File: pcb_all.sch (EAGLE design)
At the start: 1 part, among them IC1 STM32L412KBT6

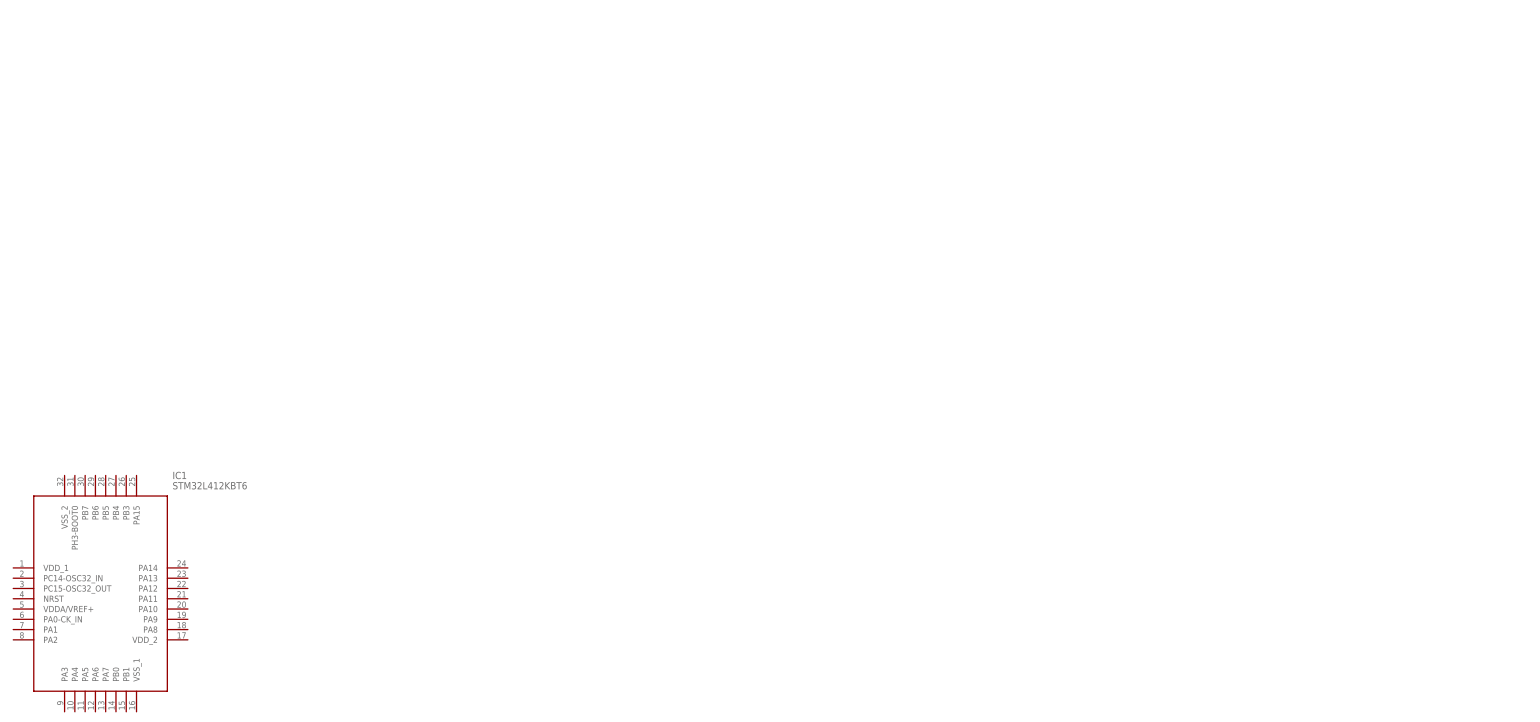
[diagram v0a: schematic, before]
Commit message: Add files via upload
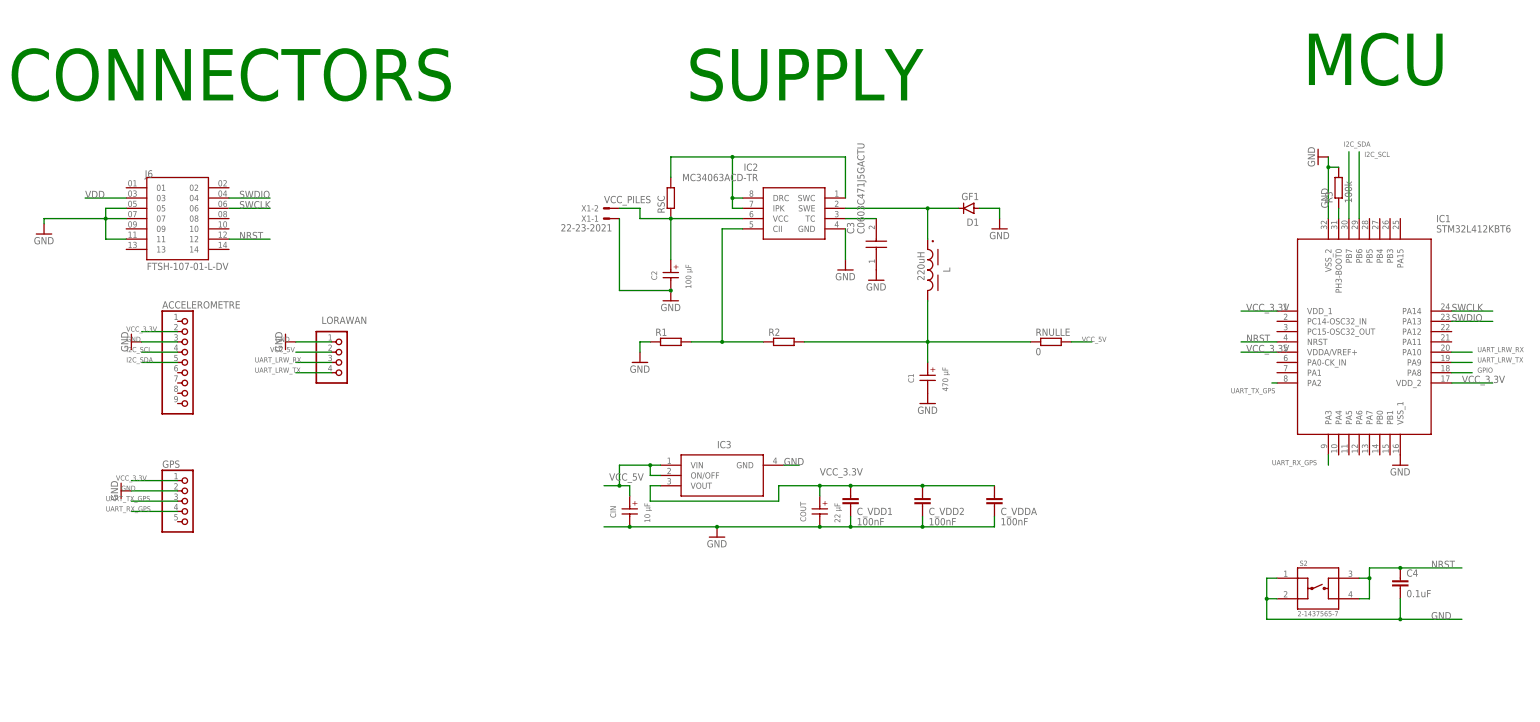
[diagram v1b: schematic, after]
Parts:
- added ACCELEROMETRE: (no value), pinhead:PINHD-1X9
- added C1: 470 µF, C1:WCAP-ASLL_8X10.5_865060353009
- added C2: 100 µF, C2:WCAP-ASLL_6.3X7.7_865060445005
- added C3: C0603C471J5GACTU, C0603C471J5GACTU:C0603C471J5GACTU
- added C4: 0.1uF, rcl:C-EUC0603
- added CIN: 10 µF, Cin:WCAP-ASLL_4X5.5_865060440001
- added COUT: 22 µF, Cout:WCAP-ASLL_5X5.5_865060442002
- added C_VDD1, C_VDD2, C_VDDA: 100nF, rcl:C-EUC0603
- added D1: GF1, diode:GF1
- added GPS: (no value), pinhead:PINHD-1X5
- added IC2: MC34063ACD-TR, SamacSys_Parts:MC34063ACD-TR
- added IC3: NCV33375ST3.3T3G, SamacSys_Parts:NCV33375ST3.3T3G
- added J6: FTSH-107-01-L-DV, FTSH-107-01-L-DV:FTSH-107-01-L-DV
- added L: 220uH, L:WE-PDA_1260_784771221
- added LORAWAN: (no value), pinhead:PINHD-1X4
- added R1, R2: (no value), rcl:R-EU_R0603
- added R3: 100k, rcl:R-EU_R0603
- added RNULLE: 0, rcl:R-EU_R0603
- added RSC: (no value), rcl:R-EU_R1206W
- added S2: 2-1437565-7, 2-1437565-7:2-1437565-7
- added X1: 22-23-2021, con-molex:22-23-2021
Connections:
- new net GND: ACCELEROMETRE.3, C1.-, C2.-, C3.1, C4.2, CIN.-, COUT.-, C_VDD1.2, C_VDD2.2, C_VDDA.2, D1.A, GPS.2, IC1.VSS_1, IC1.VSS_2, IC2.GND, IC3.GND, J6.05, J6.07, J6.11, LORAWAN.1, R1.1, R3.2, S2.1, S2.2, X1-1.S
- new net GPIO: IC1.PA8
- new net I2C_SCL: ACCELEROMETRE.4, IC1.PB6
- new net I2C_SDA: ACCELEROMETRE.5, IC1.PB7
- new net N$1: C1.+, L.2, R2.2, RNULLE.1
- new net N$2: IC2.DRC, IC2.IPK, IC2.SWC, RSC.2
- new net N$3: IC2.CII, R1.2, R2.1
- new net N$4: IC1.PH3-BOOT0, R3.1
- new net N$6: D1.C, IC2.SWE, L.1
- new net N$7: C3.2, IC2.TC
- new net NRST: C4.1, IC1.NRST, J6.12, S2.3, S2.4
- new net SWCLK: IC1.PA14, J6.06
- new net SWDIO: IC1.PA13, J6.04
- new net UART_LRW_RX: IC1.PA10, LORAWAN.3
- new net UART_LRW_TX: IC1.PA9, LORAWAN.4
- new net UART_RX_GPS: GPS.4, IC1.PA3
- new net UART_TX_GPS: GPS.3, IC1.PA2
- new net VCC_3.3V: ACCELEROMETRE.2, COUT.+, C_VDD1.1, C_VDD2.1, C_VDDA.1, GPS.1, IC1.VDDA/VREF+, IC1.VDD_1, IC1.VDD_2, IC3.VOUT
- new net VCC_5V: CIN.+, IC3.ON/OFF, IC3.VIN, LORAWAN.2, RNULLE.2
- new net VCC_PILES: C2.+, IC2.VCC, RSC.1, X1-2.S
- new net VDD: J6.03
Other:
- note added: "CONNECTORS"
- note added: "MCU"
- note added: "SUPPLY"
- moved on the sheet: IC1
